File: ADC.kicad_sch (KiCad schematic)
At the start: 7 parts, among them U7 MCP3461RT-E/NC

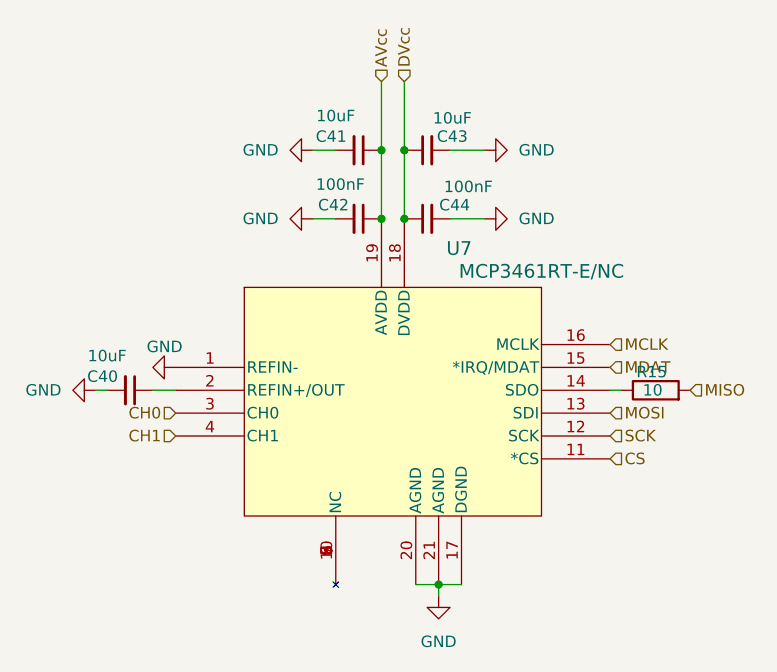
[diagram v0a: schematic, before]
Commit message: Rev 1 ready for review
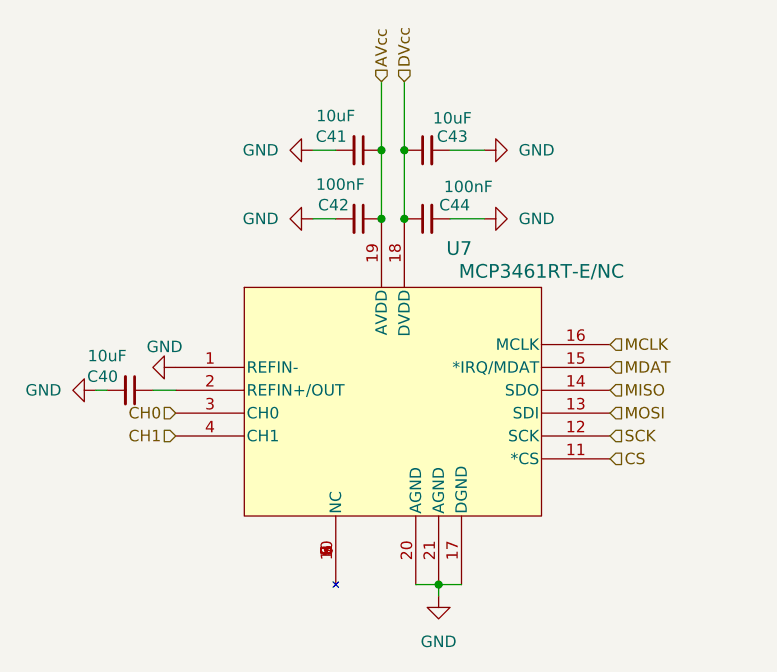
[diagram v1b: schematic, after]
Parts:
- removed R15: 10, symbol Device:R
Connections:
- net MISO: now also U7.14 (SDO)
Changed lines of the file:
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@@
-	(wire
-		(pts
-			(xy 162.56 92.71) (xy 161.29 92.71)
-		)
-		(stroke
-			(width 0)
-			(type default)
-		)
-	)
 	(wire
 		(pts
@@
 	(hierarchical_label "MISO"
 		(shape input)
-		(at 170.18 92.71 0)
+		(at 161.29 92.71 0)
 		(fields_autoplaced yes)
 		(effects
@@
 					(unit 1)
 				)
-			)
-		)
-	)
-	(symbol
-		(lib_id "Device:R")
-		(at 166.37 92.71 90)
-		(unit 1)
-		(exclude_from_sim no)
-		(in_bom yes)
-		(on_board yes)
-		(dnp no)
-		(property "Reference" "R15"
-			(at 167.64 90.678 90)
-			(effects
-				(font
-					(size 1.27 1.27)
-				)
-				(justify left)
-			)
-		)
-		(property "Value" "10"
-			(at 167.132 92.71 90)
-			(effects
-				(font
-					(size 1.27 1.27)
-				)
-				(justify left)
-			)
-		)
-		(property "Footprint" ""
-			(at 166.37 94.488 90)
-			(effects
-				(font
-					(size 1.27 1.27)
-				)
-				(hide yes)
-			)
-		)
-		(property "Datasheet" "~"
-			(at 166.37 92.71 0)
-			(effects
-				(font
-					(size 1.27 1.27)
-				)
-				(hide yes)
-			)
-		)
-		(property "Description" "Resistor"
-			(at 166.37 92.71 0)
-			(effects
-				(font
-					(size 1.27 1.27)
-				)
-				(hide yes)
-			)
-		)
-		(pin "1"
-		)
-		(pin "2"
-		)
-		(instances
-			(project "phase-detector"
-				(path "/b38ebd54-5e2b-4067-b9f0-d8faa1bf1436/2e945d6b-b9ee-4a5d-8657-99c87887e4e6"
-					(reference "R15")
-					(unit 1)
-				)
-				(path "/b38ebd54-5e2b-4067-b9f0-d8faa1bf1436/5bb5793e-cf1a-4f42-8634-782ace6b1aa8"
-					(reference "R29")
-					(unit 1)
-				)
-				(path "/b38ebd54-5e2b-4067-b9f0-d8faa1bf1436/5ddca4d8-7ba9-466f-8f9a-d6ec2c4272e5"
-					(reference "R12")
-					(unit 1)
-				)
-				(path "/b38ebd54-5e2b-4067-b9f0-d8faa1bf1436/654454e2-de4e-487a-b39e-c340ad052c70"
-					(reference "R21")
-					(unit 1)
-				)
-				(path "/b38ebd54-5e2b-4067-b9f0-d8faa1bf1436/720fc5b7-7833-4c1f-8cf6-b4c2b992425b"
-					(reference "R30")
-					(unit 1)
-				)

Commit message: moon
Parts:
- C40: footprint Capacitor_SMD:C_0402_1005Metric -> Capacitor_SMD:C_0603_1608Metric
- C41, C43: footprint Capacitor_SMD:C_0805_2012Metric -> Capacitor_SMD:C_0603_1608Metric
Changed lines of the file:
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@@
 			)
 		)
-		(property "Footprint" "Capacitor_SMD:C_0402_1005Metric"
+		(property "Footprint" "Capacitor_SMD:C_0603_1608Metric"
 			(at 107.95 92.71 0)
 			(effects
@@
 			)
 		)
-		(property "Footprint" "Capacitor_SMD:C_0805_2012Metric"
+		(property "Footprint" "Capacitor_SMD:C_0603_1608Metric"
 			(at 140.97 66.04 0)
 			(effects
@@
 			)
 		)
-		(property "Footprint" "Capacitor_SMD:C_0805_2012Metric"
+		(property "Footprint" "Capacitor_SMD:C_0603_1608Metric"
 			(at 133.35 66.04 0)
 			(effects
